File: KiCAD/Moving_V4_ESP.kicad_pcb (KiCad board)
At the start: 2 copper layers, 39 x 63 mm, 89 parts, among them J1 Vin_1, J10 IO27_GPIO1, J11 IO32_GPIO2, J12 IO5_GPIO3(PU), J2 Power_SW, J3 Vin_XT, J4 USB_B_Micro, J5 Encorder_L, J6 Encorder_R, J7 MOTOR_L, J8 MOTOR_R, J9 IO4_GPIO0, Q1 U4_ALT2, Q2 U4_ALT2, Q3 U4_ALT2, U1 CN39033A, U10 ITR8307-S17-TR8, U2 CH340X, U3 UZ1085L-33-TN3-R, U4 TXB0104RUT, U5 CP3119MDTR, U6 CP3119MDTR, U7 ESP32-WROOM-32, U8 ITR8307-S17-TR8, U9 ITR8307-S17-TR8

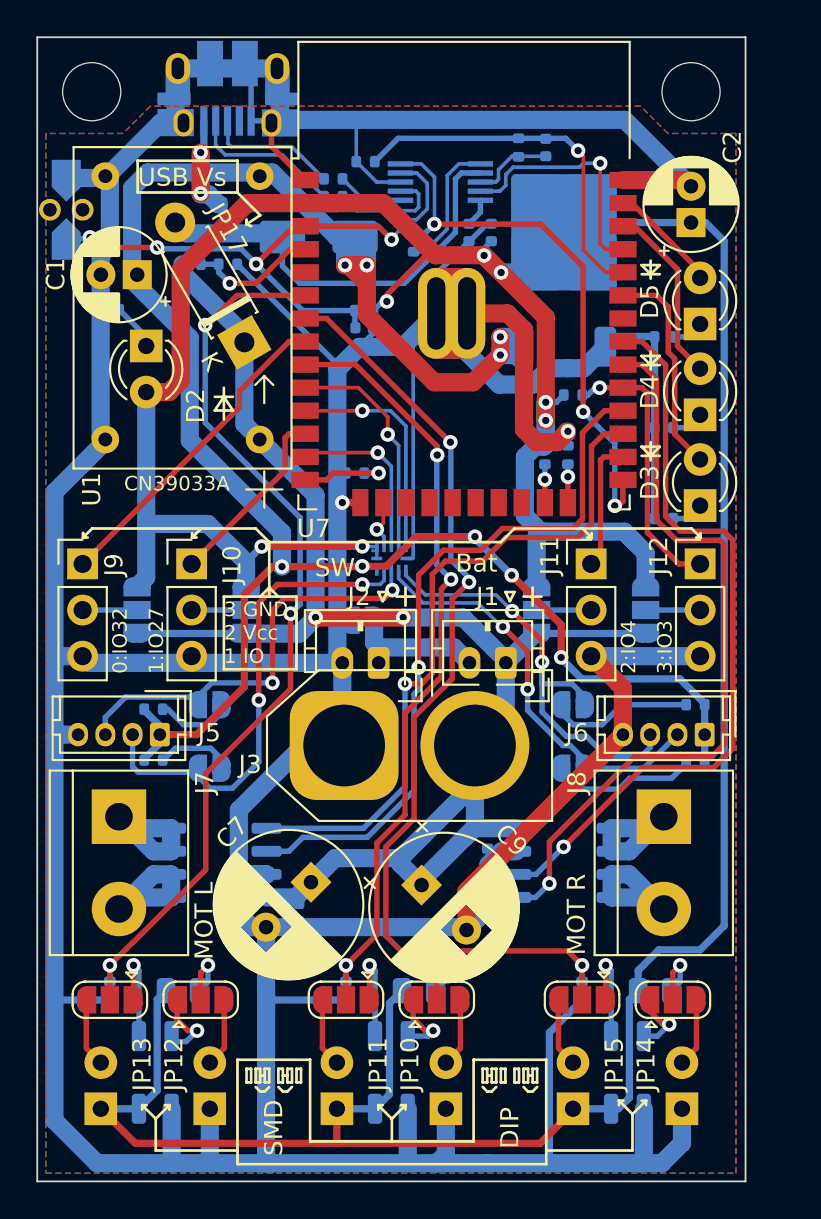
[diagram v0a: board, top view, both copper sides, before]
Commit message: 版を記入
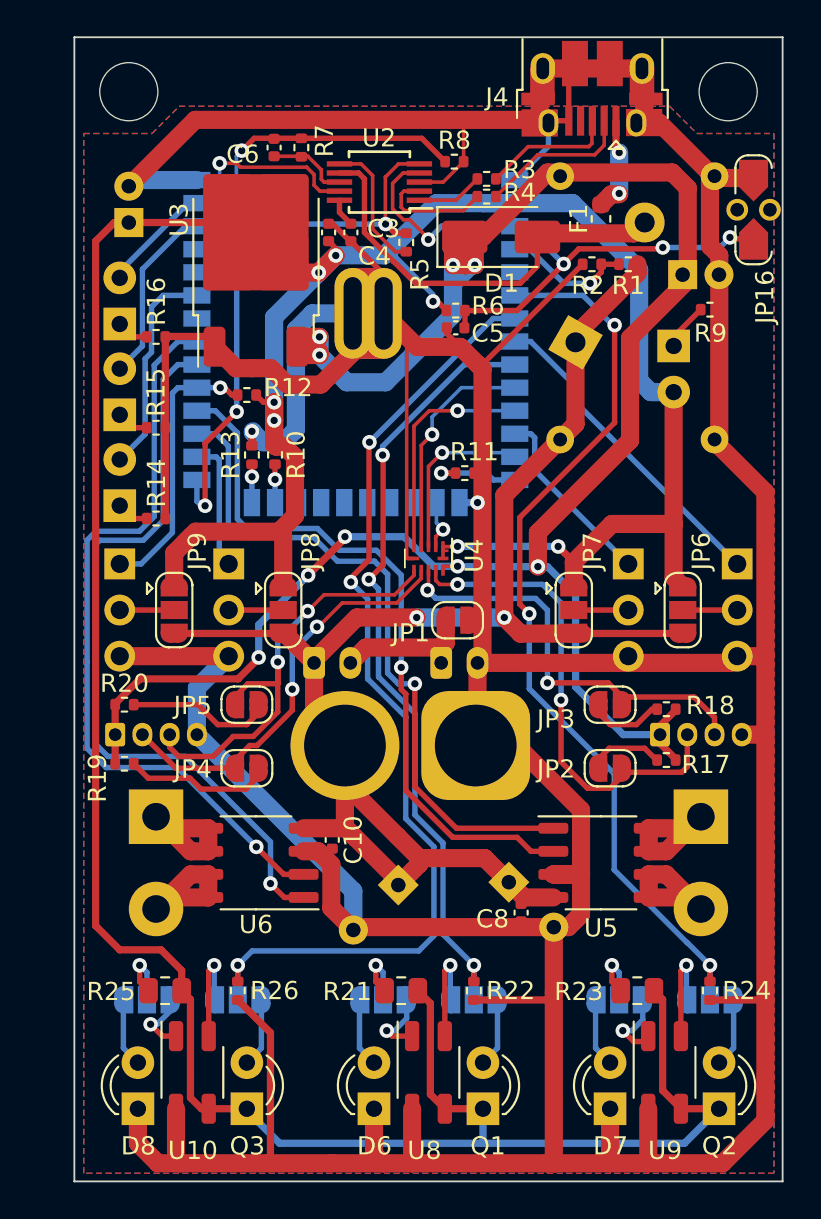
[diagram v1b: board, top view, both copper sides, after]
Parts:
- C1, C2, C7, C9, D2, D3, D4, D5, J1, J10, J11, J12, J2, J3, J5, J6, J7, J8, J9, JP10, JP11, JP12, JP13, JP14, JP15, JP17, U1, U7: moved to B.Cu
- C10, C3, C4, C5, C6, C8, D1, D6, D7, D8, F1, J4, JP1, JP16, JP2, JP3, JP4, JP5, JP6, JP7, JP8, JP9, Q1, Q2, Q3, R1, R10, R11, R12, R13, R14, R15, R16, R17, R18, R19, R2, R20, R21, R22, R23, R24, R25, R26, R3, R4, R5, R6, R7, R8, R9, REF** (x2), U10, U2, U3, U4, U5, U6, U8, U9: moved to F.Cu
- moved JP16 37.8 mm to (139.7, 109.5)
- moved J9 36.0 mm to (138.8, 129.0), turned to 180 degrees
- moved REF** 35.0 mm to (138.3, 103.0), turned to 0 degrees
- moved Q2 34.0 mm to (137.8, 159.0)
- moved JP13 33.0 mm to (137.3, 153.0), turned to 0 degrees
- moved R24 33.0 mm to (137.3, 152.5)
- moved R9 33.0 mm to (137.3, 115.0), turned to 0 degrees
- moved J6 32.5 mm to (104.5, 138.4), turned to 0 degrees
- moved J7 32.0 mm to (136.8, 142.9)
- moved D3 32.0 mm to (104.8, 125.8)
- moved D4 32.0 mm to (104.8, 120.8)
- moved D5 32.0 mm to (104.8, 115.8)
- moved J12 32.0 mm to (104.8, 129.0), turned to 180 degrees
- moved R19 31.4 mm to (105.1, 140.0), turned to 0 degrees
- moved R20 31.4 mm to (105.1, 136.8), turned to 0 degrees
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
